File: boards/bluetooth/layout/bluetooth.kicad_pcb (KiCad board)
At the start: 2 copper layers, 16 x 25 mm, 9 parts, among them U1 HM-19

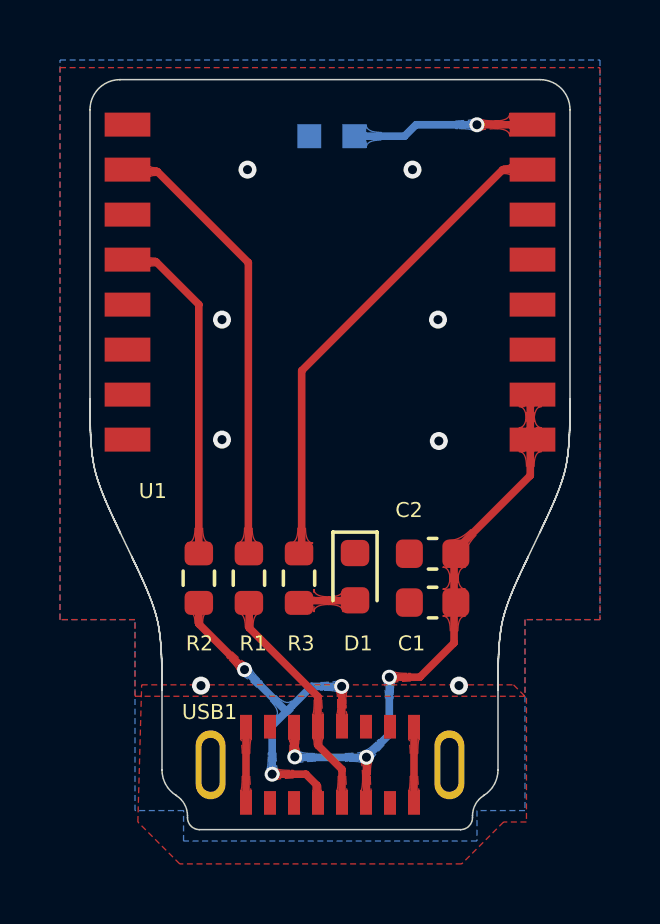
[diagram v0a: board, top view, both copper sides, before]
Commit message: 🚚 Transfer the Altium pour, teardrop and outline settings to the layouts
The transfer scripts now carry what KiCad's Altium importer drops, and
the layouts are regenerated with them:

- Teardrops (converted to plain zones) fill with a 0.1 mm minimum width
  instead of the importer's 0.25 mm, which left 652 of 786 (main), 5 of
  25 (encoder) and 10 of 46 (bluetooth) teardrops without copper. 0.1 mm
  is JLCPCB's minimum copper feature: 0.0254 mm fills slightly more but
  fails the DFM feature width on all three boards.
- Pours use the Altium polygons' neck width as minimum width (0.1 mm;
  0.4 mm on the encoder's bottom pour, which keeps it out of the channels
  between the SPI tracks, 0.3 mm on the bluetooth plug pour).
- Inner-layer pours relieve through-hole pads (0.254 mm spokes and gap,
  Altium rule PolygonConnect); outer pours stay solid.
- Main In1/In2 keep Altium's 1.559 / 2.074 mm voids around H1-H4
  (copper-pour keepouts).
- Edge.Cuts lines under 1 um (main 6, encoder 1, bluetooth 7) are left
  out and their neighbours joined, so KiCad reads the outlines as valid.
- The board mask expansion is copied from the previous board (0.02 mm);
  main takes the spec's aux origin.
- D4/D5 and bluetooth D1 3D models are scaled to the datasheet heights.
- rework.py catches all six teardrops of the removed C1 VBAT chain (three
  were left as stubs, invisible while unfilled).
- The encoder drops an embedded TSSOP-14 STEP no footprint uses; the
  bluetooth script calls previous.altium_pcb (renamed).

The main layout footprints were resynced from their packages
(pcb layout --sync-footprints), which brings the new WallSensor
silkscreen, R31-R33 and U2's keepouts on all four copper layers.
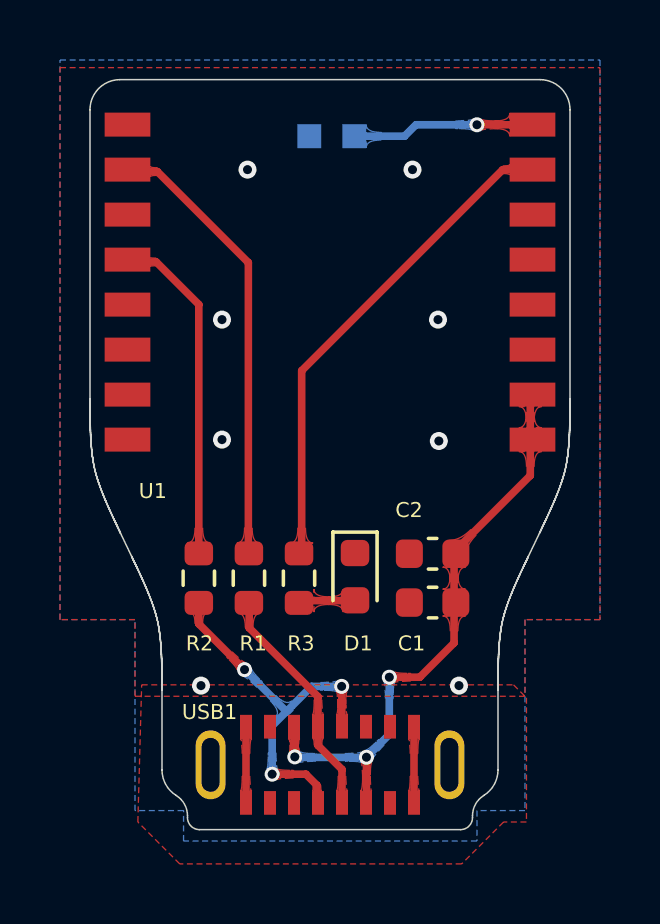
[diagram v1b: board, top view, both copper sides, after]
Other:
- outline, holes or cut-outs redrawn
- rule pad_to_mask_clearance: 0 -> 0.02
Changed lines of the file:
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@@
 			(dielectric_constraints no)
 		)
-		(pad_to_mask_clearance 0)
+		(pad_to_mask_clearance 0.02)
 		(allow_soldermask_bridges_in_footprints no)
 		(tenting
@@
 			)
 			(scale
-				(xyz 1 1 1)
+				(xyz 1 1 0.5)
 			)
 			(rotate
@@
 	(gr_line
 		(start 141.501094 92.503595)
-		(end 141.501095 92.503595)
-		(stroke
-			(width 0.05)
-			(type solid)
-		)
-		(layer "Edge.Cuts")
-	)
-	(gr_line
-		(start 141.501095 92.503595)
 		(end 155.501105 92.503595)
 		(stroke
@@
 	)
 	(gr_line
-		(start 142.901095 115.514905)
-		(end 142.901095 112.847575)
-		(stroke
-			(width 0.05)
-			(type solid)
-		)
-		(layer "Edge.Cuts")
-	)
-	(gr_line
 		(start 142.901095 115.514906)
-		(end 142.901095 115.514905)
+		(end 142.901095 112.847575)
 		(stroke
 			(width 0.05)
@@
 	)
 	(gr_arc
-		(start 143.373321 116.36429)
+		(start 143.373319 116.36429)
 		(mid 143.027089 116.00082)
 		(end 142.901095 115.514906)
@@
 		(layer "Edge.Cuts")
 	)
-	(gr_line
-		(start 143.373319 116.36429)
-		(end 143.373321 116.36429)
-		(stroke
-			(width 0.05)
-			(type solid)
-		)
-		(layer "Edge.Cuts")
-	)
 	(gr_arc
 		(start 143.373319 116.36429)
@@
 	(gr_line
 		(start 143.751095 117.103595)
-		(end 143.751105 117.103595)
-		(stroke
-			(width 0.05)
-			(type solid)
-		)
-		(layer "Edge.Cuts")
-	)
-	(gr_line
-		(start 143.751105 117.103595)
 		(end 143.751095 117.043797)
 		(stroke
@@
 	)
 	(gr_line
-		(start 152.851095 117.503595)
-		(end 144.151095 117.503595)
-		(stroke
-			(width 0.05)
-			(type solid)
-		)
-		(layer "Edge.Cuts")
-	)
-	(gr_line
 		(start 152.851094 117.503595)
-		(end 152.851095 117.503595)
-		(stroke
-			(width 0.05)
-			(type solid)
-		)
-		(layer "Edge.Cuts")
-	)
-	(gr_line
-		(start 153.251095 117.043795)
-		(end 153.251095 117.103596)
+		(end 144.151095 117.503595)
 		(stroke
 			(width 0.05)
@@
 	(gr_line
 		(start 153.251105 117.043798)
-		(end 153.251095 117.043795)
+		(end 153.251095 117.103596)
 		(stroke
 			(width 0.05)
@@
 		(start 153.251105 117.043798)
 		(mid 153.351908 116.655076)
-		(end 153.628885 116.364298)
-		(stroke
-			(width 0.05)
-			(type solid)
-		)
-		(layer "Edge.Cuts")
-	)
-	(gr_line
-		(start 153.628876 116.36429)
-		(end 153.628885 116.364298)
+		(end 153.628876 116.36429)
 		(stroke
 			(width 0.05)
@@
 			(clearance 0.1)
 		)
-		(min_thickness 0.25)
+		(min_thickness 0.1)
 		(fill yes
 			(thermal_gap 0.5)
@@
 			(clearance 0.1)
 		)
-		(min_thickness 0.25)
+		(min_thickness 0.1)
 		(fill yes
 			(thermal_gap 0.5)
@@
 			(clearance 0.1)
 		)
-		(min_thickness 0.25)
+		(min_thickness 0.1)
 		(fill yes
 			(thermal_gap 0.5)
@@
 			(clearance 0.1)
 		)
-		(min_thickness 0.25)
+		(min_thickness 0.1)
 		(fill yes
 			(thermal_gap 0.5)
@@
 			(clearance 0.1)
 		)
-		(min_thickness 0.25)
+		(min_thickness 0.1)
 		(fill yes
 			(thermal_gap 0.5)
@@
 			(clearance 0.1)
 		)
-		(min_thickness 0.25)
+		(min_thickness 0.1)
 		(fill yes
 			(thermal_gap 0.5)
@@
 			(clearance 0.1)
 		)
-		(min_thickness 0.25)
+		(min_thickness 0.1)
 		(fill yes
 			(thermal_gap 0.5)
@@
 			(clearance 0.1)
 		)
-		(min_thickness 0.25)
+		(min_thickness 0.1)
 		(fill yes
 			(thermal_gap 0.5)
@@
 			(clearance 0.1)
 		)
-		(min_thickness 0.25)
+		(min_thickness 0.3)
 		(fill yes
 			(thermal_gap 0.254)
@@
 			(clearance 0.1)
 		)
-		(min_thickness 0.25)
+		(min_thickness 0.1)
 		(fill yes
 			(thermal_gap 0.5)
@@
 			(clearance 0.1)
 		)
-		(min_thickness 0.25)
+		(min_thickness 0.1)
 		(fill yes
 			(thermal_gap 0.5)
@@
 			(clearance 0.1)
 		)
-		(min_thickness 0.25)
+		(min_thickness 0.1)
 		(fill yes
 			(thermal_gap 0.5)
@@
 			(clearance 0.1)
 		)
-		(min_thickness 0.25)
+		(min_thickness 0.1)
 		(fill yes
 			(thermal_gap 0.5)
@@
 			(clearance 0.1)
 		)
-		(min_thickness 0.25)
+		(min_thickness 0.1)
 		(fill yes
 			(thermal_gap 0.5)
@@
 			(clearance 0.1)
 		)
-		(min_thickness 0.25)
+		(min_thickness 0.1)
 		(fill yes
 			(thermal_gap 0.5)
@@
 			(clearance 0.1)
 		)
-		(min_thickness 0.25)
+		(min_thickness 0.1)
 		(fill yes
 			(thermal_gap 0.5)
@@
 			(clearance 0.1)
 		)
-		(min_thickness 0.25)
+		(min_thickness 0.1)
 		(fill yes
 			(thermal_gap 0.5)
@@
 			(clearance 0.1)
 		)
-		(min_thickness 0.25)
+		(min_thickness 0.1)
 		(fill yes
 			(thermal_gap 0.5)
@@
 			(clearance 0.1)
 		)
-		(min_thickness 0.25)
+		(min_thickness 0.1)
 		(fill yes
 			(thermal_gap 0.5)
@@
 			(clearance 0.1)
 		)
-		(min_thickness 0.25)
+		(min_thickness 0.1)
 		(fill yes
 			(thermal_gap 0.5)
@@
 			(clearance 0.1)
 		)
-		(min_thickness 0.25)
+		(min_thickness 0.1)
 		(fill yes
 			(thermal_gap 0.5)
@@
 			(clearance 0.1)
 		)
-		(min_thickness 0.25)
+		(min_thickness 0.1)
 		(fill yes
 			(thermal_gap 0.5)
@@
 			(clearance 0.1)
 		)
-		(min_thickness 0.25)
+		(min_thickness 0.1)
 		(fill yes
 			(thermal_gap 0.5)
@@
 			(clearance 0.1)
 		)
-		(min_thickness 0.25)
+		(min_thickness 0.1)
 		(fill yes
 			(thermal_gap 0.5)
@@
 			(clearance 0.1)
 		)
-		(min_thickness 0.25)
+		(min_thickness 0.1)
 		(fill yes
 			(thermal_gap 0.5)
@@
 			(clearance 0.1)
 		)
-		(min_thickness 0.25)
+		(min_thickness 0.1)
 		(fill yes
 			(thermal_gap 0.254)
@@
 			(clearance 0.1)
 		)
-		(min_thickness 0.25)
+		(min_thickness 0.1)
 		(fill yes
 			(thermal_gap 0.5)
@@
 			(clearance 0.1)
 		)
-		(min_thickness 0.25)
+		(min_thickness 0.1)
 		(fill yes
 			(thermal_gap 0.5)
@@
 			(clearance 0.1)
 		)
-		(min_thickness 0.25)
+		(min_thickness 0.1)
 		(fill yes
 			(thermal_gap 0.5)
@@
 			(clearance 0.1)
 		)
-		(min_thickness 0.25)
+		(min_thickness 0.1)
 		(fill yes
 			(thermal_gap 0.5)
@@
 			(clearance 0.1)
 		)
-		(min_thickness 0.25)
+		(min_thickness 0.1)
 		(fill yes
 			(thermal_gap 0.5)
@@
 			(clearance 0.1)
 		)
-		(min_thickness 0.25)
+		(min_thickness 0.1)
 		(fill yes
 			(thermal_gap 0.5)
@@
 			(clearance 0.1)
 		)
-		(min_thickness 0.25)
+		(min_thickness 0.1)
 		(fill yes
 			(thermal_gap 0.5)
@@
 			(clearance 0.1)
 		)
-		(min_thickness 0.25)
+		(min_thickness 0.1)
 		(fill yes
 			(thermal_gap 0.5)
@@
 			(clearance 0.1)
 		)
-		(min_thickness 0.25)
+		(min_thickness 0.1)
 		(fill yes
 			(thermal_gap 0.5)
@@
 			(clearance 0.1)
 		)
-		(min_thickness 0.25)
+		(min_thickness 0.1)
 		(fill yes
 			(thermal_gap 0.5)
@@
 			(clearance 0.1)
 		)
-		(min_thickness 0.25)
+		(min_thickness 0.1)
 		(fill yes
 			(thermal_gap 0.5)
@@
 			(clearance 0.1)
 		)
-		(min_thickness 0.25)
+		(min_thickness 0.1)
 		(fill yes
 			(thermal_gap 0.5)
@@
 			(clearance 0.1)
 		)
-		(min_thickness 0.25)
+		(min_thickness 0.1)
 		(fill yes
 			(thermal_gap 0.5)
@@
 			(clearance 0.1)
 		)
-		(min_thickness 0.25)
+		(min_thickness 0.1)
 		(fill yes
 			(thermal_gap 0.254)
@@
 			(clearance 0.1)
 		)
-		(min_thickness 0.25)
+		(min_thickness 0.1)
 		(fill yes
 			(thermal_gap 0.5)
@@
 			(clearance 0.1)
 		)
-		(min_thickness 0.25)
+		(min_thickness 0.1)
 		(fill yes
 			(thermal_gap 0.5)
@@
 			(clearance 0.1)
 		)
-		(min_thickness 0.25)
+		(min_thickness 0.1)
 		(fill yes
 			(thermal_gap 0.5)
@@
 			(clearance 0.1)
 		)
-		(min_thickness 0.25)
+		(min_thickness 0.1)
 		(fill yes
 			(thermal_gap 0.5)
@@
 			(clearance 0.1)
 		)
-		(min_thickness 0.25)
+		(min_thickness 0.1)
 		(fill yes
 			(thermal_gap 0.5)
@@
 			(clearance 0.1)
 		)
-		(min_thickness 0.25)
+		(min_thickness 0.1)
 		(fill yes
 			(thermal_gap 0.5)
@@
 			(clearance 0.1)
 		)
-		(min_thickness 0.25)
+		(min_thickness 0.1)
 		(fill yes
 			(thermal_gap 0.5)
@@
 			(clearance 0.1)
 		)
-		(min_thickness 0.25)
+		(min_thickness 0.1)
 		(fill yes
 			(thermal_gap 0.5)
@@
 			(clearance 0.1)
 		)
-		(min_thickness 0.25)
+		(min_thickness 0.1)
 		(fill yes
 			(thermal_gap 0.5)
